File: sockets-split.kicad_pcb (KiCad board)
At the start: 2 copper layers, 63 parts, among them J2 MJ-4PP-9, P1 i2c-pin, P2 i2c-pin, SW1 RESET_SW, SW10 SW_PUSH, SW11 SW_PUSH, SW12 SW_PUSH, SW13 SW_PUSH, SW14 SW_PUSH, SW15 SW_PUSH, SW16 SW_PUSH, SW17 SW_PUSH, SW18 SW_PUSH, SW19 SW_PUSH, SW2 SW_PUSH, SW20 SW_PUSH, SW21 SW_PUSH, SW22 SW_PUSH, SW23 SW_PUSH, SW24 SW_PUSH, SW25 SW_PUSH, SW3 SW_PUSH, SW4 SW_PUSH, SW5 SW_PUSH, SW6 SW_PUSH, SW7 SW_PUSH, SW8 SW_PUSH, SW9 SW_PUSH, U1 ProMicro

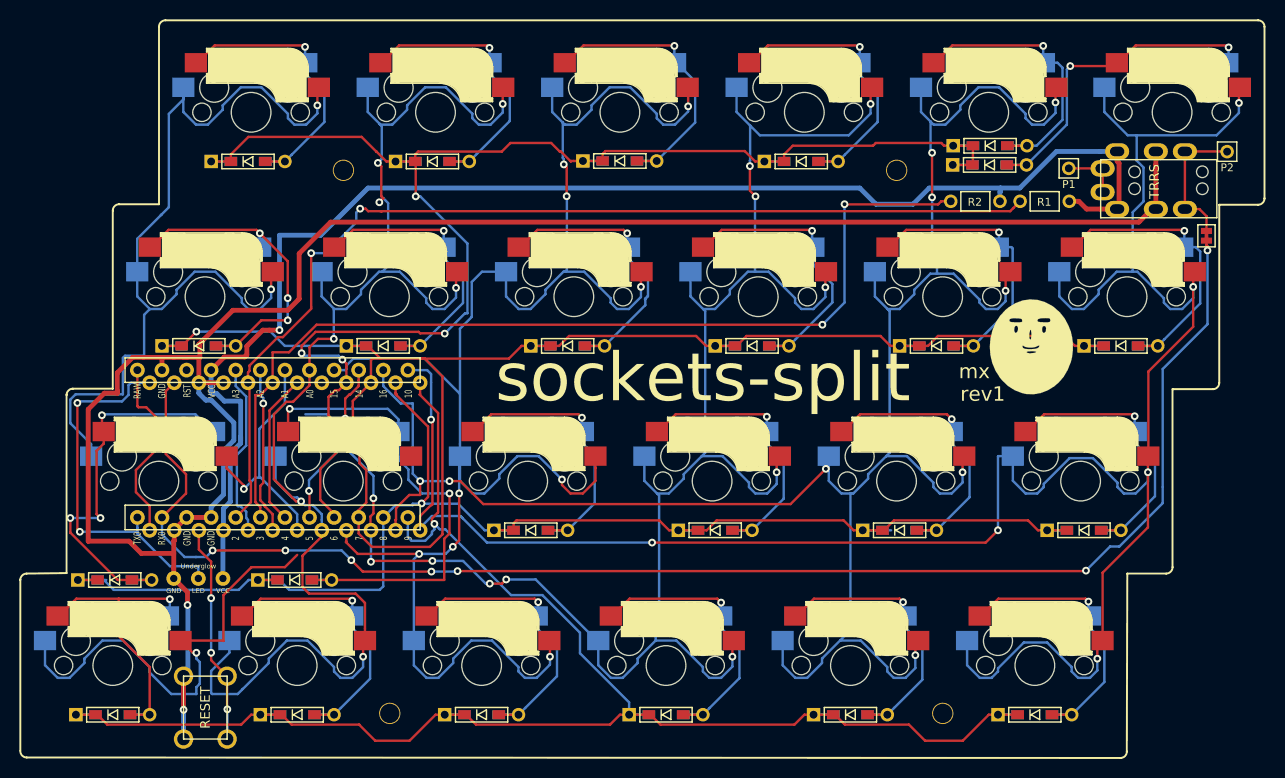
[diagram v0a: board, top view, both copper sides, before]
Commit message: Fix promicro, case
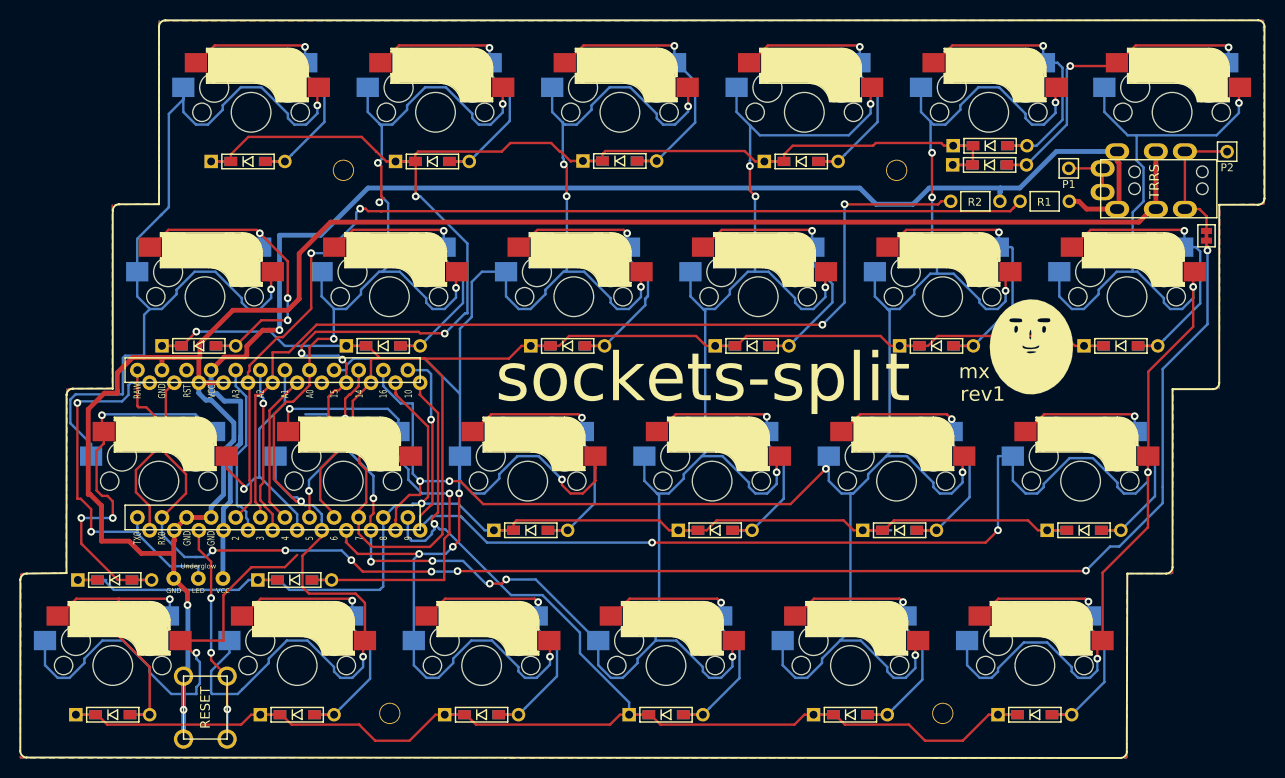
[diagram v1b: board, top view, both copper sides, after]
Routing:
- net GND: track 205.7 -> 205.0 mm
- added copper zone on B.Cu, net GND
- added copper zone on F.Cu, net GND
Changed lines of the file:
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@@
     (thickness 1.6)
     (drawings 161)
-    (tracks 1485)
+    (tracks 1492)
     (zones 0)
     (modules 63)
@@
     (0 F.Cu signal)
     (31 B.Cu signal)
-    (32 B.Adhes user)
-    (33 F.Adhes user)
-    (34 B.Paste user)
-    (35 F.Paste user)
+    (32 B.Adhes user hide)
+    (33 F.Adhes user hide)
+    (34 B.Paste user hide)
+    (35 F.Paste user hide)
     (36 B.SilkS user)
     (37 F.SilkS user)
@@
     (39 F.Mask user)
     (40 Dwgs.User user)
-    (41 Cmts.User user)
-    (42 Eco1.User user)
-    (43 Eco2.User user)
-    (44 Edge.Cuts user)
-    (45 Margin user)
-    (46 B.CrtYd user)
+    (41 Cmts.User user hide)
+    (42 Eco1.User user hide)
+    (43 Eco2.User user hide)
+    (44 Edge.Cuts user hide)
+    (45 Margin user hide)
+    (46 B.CrtYd user hide)
     (47 F.CrtYd user hide)
-    (48 B.Fab user)
-    (49 F.Fab user)
+    (48 B.Fab user hide)
+    (49 F.Fab user hide)
   )
   (setup
@@
     (visible_elements 7FFFE7FF)
     (pcbplotparams
-      (layerselection 0x00100_7ffffffe)
+      (layerselection 0x010f0_ffffffff)
       (usegerberextensions false)
       (usegerberattributes false)
@@
       (padsonsilk false)
       (subtractmaskfromsilk false)
-      (outputformat 3)
+      (outputformat 1)
       (mirror false)
       (drillshape 0)
@@
   (segment (start 102.5622 109.7788) (end 104.5972 109.7788) (width 0.25) (layer B.Cu) (net 15))
   (segment (start 102.5622 109.7788) (end 104.5972 109.7788) (width 0.25) (layer F.Cu) (net 15))
-  (via (at 96.2014 103.378) (size 0.8) (drill 0.4) (layers F.Cu B.Cu) (net 15))
-  (segment (start 96.2014 104.894402) (end 96.2014 103.378) (width 0.25) (layer F.Cu) (net 15))
-  (via (at 99.314 103.378) (size 0.8) (drill 0.4) (layers F.Cu B.Cu) (net 15))
-  (segment (start 96.2014 103.378) (end 99.314 103.378) (width 0.25) (layer B.Cu) (net 15))
+  (via (at 97.3328 103.378) (size 0.8) (drill 0.4) (layers F.Cu B.Cu) (net 15))
+  (via (at 100.584 103.378) (size 0.8) (drill 0.4) (layers F.Cu B.Cu) (net 15))
+  (segment (start 97.4344 103.378) (end 100.547 103.378) (width 0.25) (layer B.Cu) (net 15))
   (segment (start 99.6465 95.698) (end 99.6465 94.448) (width 0.25) (layer F.Cu) (net 15))
   (segment (start 98.914001 96.430499) (end 99.6465 95.698) (width 0.25) (layer F.Cu) (net 15))
-  (segment (start 98.914001 102.978001) (end 98.914001 96.430499) (width 0.25) (layer F.Cu) (net 15))
-  (segment (start 99.314 103.378) (end 98.914001 102.978001) (width 0.25) (layer F.Cu) (net 15))
-  (segment (start 96.2014 104.894402) (end 96.207602 104.894402) (width 0.25) (layer F.Cu) (net 15))
   (segment (start 101.092 109.7788) (end 102.5622 109.7788) (width 0.25) (layer F.Cu) (net 15))
-  (segment (start 96.207602 104.894402) (end 101.092 109.7788) (width 0.25) (layer F.Cu) (net 15))
+  (segment (start 98.914001 100.5332) (end 99.472801 101.092) (width 0.25) (layer F.Cu) (net 15))
+  (segment (start 98.914001 100.5332) (end 98.914001 96.430499) (width 0.25) (layer F.Cu) (net 15))
+  (segment (start 99.472801 101.092) (end 100.0252 101.092) (width 0.25) (layer F.Cu) (net 15))
+  (segment (start 100.584 101.6508) (end 100.584 103.378) (width 0.25) (layer F.Cu) (net 15))
+  (segment (start 100.0252 101.092) (end 100.584 101.6508) (width 0.25) (layer F.Cu) (net 15))
+  (segment (start 97.3328 106.0196) (end 97.4344 106.1212) (width 0.25) (layer F.Cu) (net 15))
+  (segment (start 97.3328 103.378) (end 97.3328 106.0196) (width 0.25) (layer F.Cu) (net 15))
+  (segment (start 97.4344 106.1212) (end 101.092 109.7788) (width 0.25) (layer F.Cu) (net 15))
   (segment (start 96.9772 109.7788) (end 99.0122 109.7788) (width 0.25) (layer B.Cu) (net 16))
   (segment (start 115.57 109.7788) (end 117.605 109.7788) (width 0.25) (layer B.Cu) (net 16))
@@
   (segment (start 112.725199 96.723201) (end 112.8268 96.6216) (width 0.5) (layer B.Cu) (net 29))
   (via (at 96.9264 91.4908) (size 0.8) (drill 0.4) (layers F.Cu B.Cu) (net 30))
-  (via (at 97.1804 104.8004) (size 0.8) (drill 0.4) (layers F.Cu B.Cu) (net 30))
-  (segment (start 96.9264 91.4908) (end 96.9264 104.5464) (width 0.25) (layer F.Cu) (net 30))
-  (segment (start 96.9264 104.5464) (end 97.1804 104.8004) (width 0.25) (layer F.Cu) (net 30))
+  (via (at 98.3488 104.8004) (size 0.8) (drill 0.4) (layers F.Cu B.Cu) (net 30))
   (segment (start 109.4232 109.6264) (end 109.4232 108.3564) (width 0.25) (layer B.Cu) (net 30))
   (segment (start 103.124 104.39923) (end 103.124 104.8004) (width 0.25) (layer B.Cu) (net 30))
   (segment (start 103.124 103.3216) (end 103.124 104.39923) (width 0.25) (layer B.Cu) (net 30))
-  (segment (start 97.1804 104.8004) (end 103.124 104.8004) (width 0.25) (layer B.Cu) (net 30))
   (segment (start 106.493638 108.3564) (end 109.4232 108.3564) (width 0.25) (layer B.Cu) (net 30))
   (segment (start 103.124 104.986762) (end 106.493638 108.3564) (width 0.25) (layer B.Cu) (net 30))
@@
   (segment (start 96.9264 91.4908) (end 97.08804 91.32916) (width 0.25) (layer B.Cu) (net 30))
   (segment (start 97.08804 91.32916) (end 101.539168 91.32916) (width 0.25) (layer B.Cu) (net 30))
+  (segment (start 96.9264 101.3968) (end 97.282 101.3968) (width 0.25) (layer F.Cu) (net 30))
+  (segment (start 96.9264 91.4908) (end 96.9264 101.3968) (width 0.25) (layer F.Cu) (net 30))
+  (segment (start 98.3488 102.4636) (end 98.3488 104.8004) (width 0.25) (layer F.Cu) (net 30))
+  (segment (start 97.282 101.3968) (end 98.3488 102.4636) (width 0.25) (layer F.Cu) (net 30))
+  (segment (start 98.3488 104.8004) (end 103.124 104.8004) (width 0.25) (layer B.Cu) (net 30))
   (segment (start 111.9124 89.931762) (end 111.9124 89.17923) (width 0.5) (layer B.Cu) (net 31))
   (segment (start 208.8896 71.226601) (end 208.4488 71.667401) (width 0.5) (layer F.Cu) (net 31))
@@
   (segment (start 107.8992 126.209919) (end 107.893471 126.215648) (width 0.5) (layer B.Cu) (net 31))
   (segment (start 107.8992 123.19) (end 107.8992 126.209919) (width 0.5) (layer B.Cu) (net 31))
-  (segment (start 98.056197 105.758401) (end 98.046499 105.768099) (width 0.5) (layer F.Cu) (net 31))
-  (segment (start 98.046499 105.768099) (end 98.046499 92.148701) (width 0.5) (layer F.Cu) (net 31))
   (segment (start 99.716041 90.479159) (end 101.050855 90.479159) (width 0.5) (layer F.Cu) (net 31))
   (segment (start 98.046499 92.148701) (end 99.716041 90.479159) (width 0.5) (layer F.Cu) (net 31))
@@
   (segment (start 110.744 102.24397) (end 112.025189 100.962781) (width 0.5) (layer B.Cu) (net 31))
   (segment (start 110.744 103.3216) (end 110.744 102.24397) (width 0.5) (layer B.Cu) (net 31))
-  (segment (start 98.046499 105.768099) (end 102.262899 105.768099) (width 0.5) (layer F.Cu) (net 31))
   (segment (start 103.5304 107.0356) (end 106.8832 107.0356) (width 0.5) (layer F.Cu) (net 31))
   (segment (start 102.262899 105.768099) (end 103.5304 107.0356) (width 0.5) (layer F.Cu) (net 31))
   (segment (start 106.8832 108.54877) (end 106.8832 107.0356) (width 0.5) (layer F.Cu) (net 31))
   (segment (start 106.8832 107.0356) (end 106.8832 105.758401) (width 0.5) (layer F.Cu) (net 31))
+  (segment (start 98.046499 100.9396) (end 98.2472 100.9396) (width 0.5) (layer F.Cu) (net 31))
+  (segment (start 98.046499 100.9396) (end 98.046499 92.148701) (width 0.5) (layer F.Cu) (net 31))
+  (segment (start 99.4156 102.108) (end 99.4156 105.768099) (width 0.5) (layer F.Cu) (net 31))
+  (segment (start 98.2472 100.9396) (end 99.4156 102.108) (width 0.5) (layer F.Cu) (net 31))
+  (segment (start 99.4156 105.768099) (end 102.262899 105.768099) (width 0.5) (layer F.Cu) (net 31))
   (via (at 110.8964 106.7308) (size 0.8) (drill 0.4) (layers F.Cu B.Cu) (net 32))
   (via (at 118.4148 106.7308) (size 0.8) (drill 0.4) (layers F.Cu B.Cu) (net 32))
@@
   (segment (start 212.834 71.464201) (end 213.5632 72.193401) (width 0.25) (layer F.Cu) (net 48))
   (segment (start 211.334 71.464201) (end 212.834 71.464201) (width 0.25) (layer F.Cu) (net 48))
+  (zone (net 31) (net_name GND) (layer F.Cu) (hatch edge 0.508)
+    (connect_pads (clearance 0.508))
+    (min_thickness 0.254)
+    (fill yes (arc_segments 16) (thermal_gap 0.508) (thermal_bridge_width 0.508))
+    (polygon
+      (pts
+        (xy 105.3592 52.0192) (xy 105.3592 70.9168) (xy 100.5332 71.0184) (xy 100.5332 89.9668) (xy 95.8596 90.0176)
+        (xy 95.758 109.0676) (xy 91.0844 109.1184) (xy 91.0336 128.1684) (xy 205.3336 128.1684) (xy 205.3844 109.1184)
+        (xy 210.058 109.1184) (xy 210.1088 90.0684) (xy 214.884 90.0176) (xy 214.9348 71.0184) (xy 219.5068 70.9676)
+        (xy 219.456 51.9684)
+      )
+    )
+  )
+  (zone (net 31) (net_name GND) (layer B.Cu) (hatch edge 0.508)
+    (connect_pads (clearance 0.508))
+    (min_thickness 0.254)
+    (fill yes (arc_segments 16) (thermal_gap 0.508) (thermal_bridge_width 0.508))
+    (polygon
+      (pts
+        (xy 105.3592 52.0192) (xy 105.3592 70.9168) (xy 100.5332 71.0184) (xy 100.5332 89.9668) (xy 95.8596 90.0176)
+        (xy 95.758 109.0676) (xy 91.0844 109.1184) (xy 91.0336 128.1684) (xy 205.3336 128.1684) (xy 205.3844 109.1184)
+        (xy 210.058 109.1184) (xy 210.1088 90.0684) (xy 214.884 90.0176) (xy 214.9348 71.0184) (xy 219.5068 70.9676)
+        (xy 219.456 51.9684)
+      )
+    )
+  )
 )
